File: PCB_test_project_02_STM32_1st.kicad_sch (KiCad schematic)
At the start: 12 parts

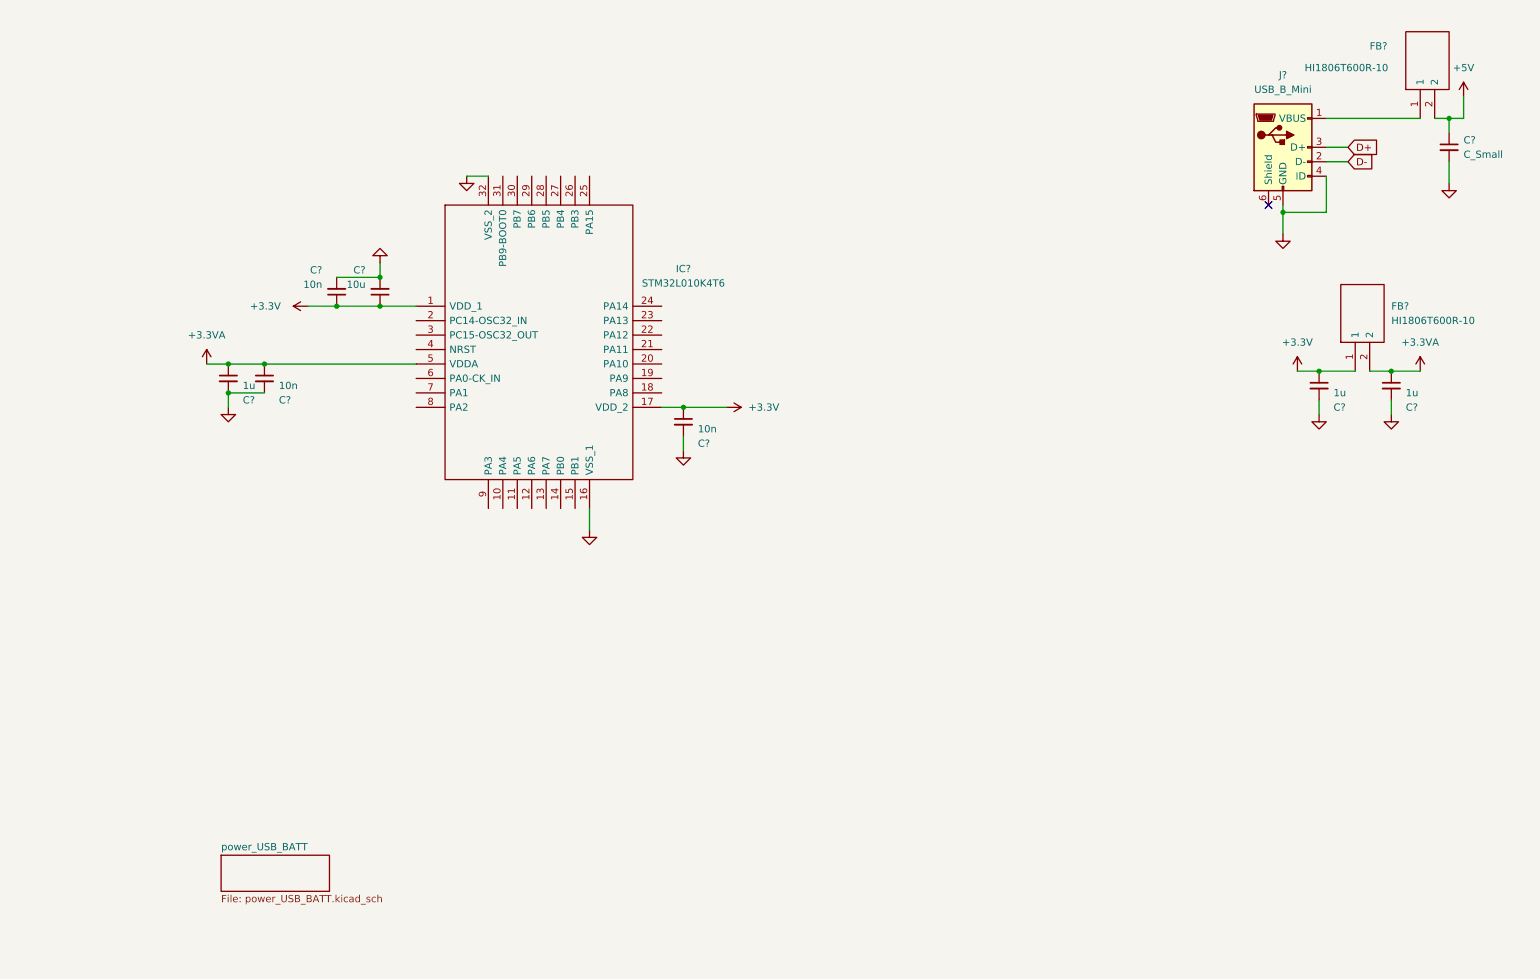
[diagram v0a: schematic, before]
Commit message: b
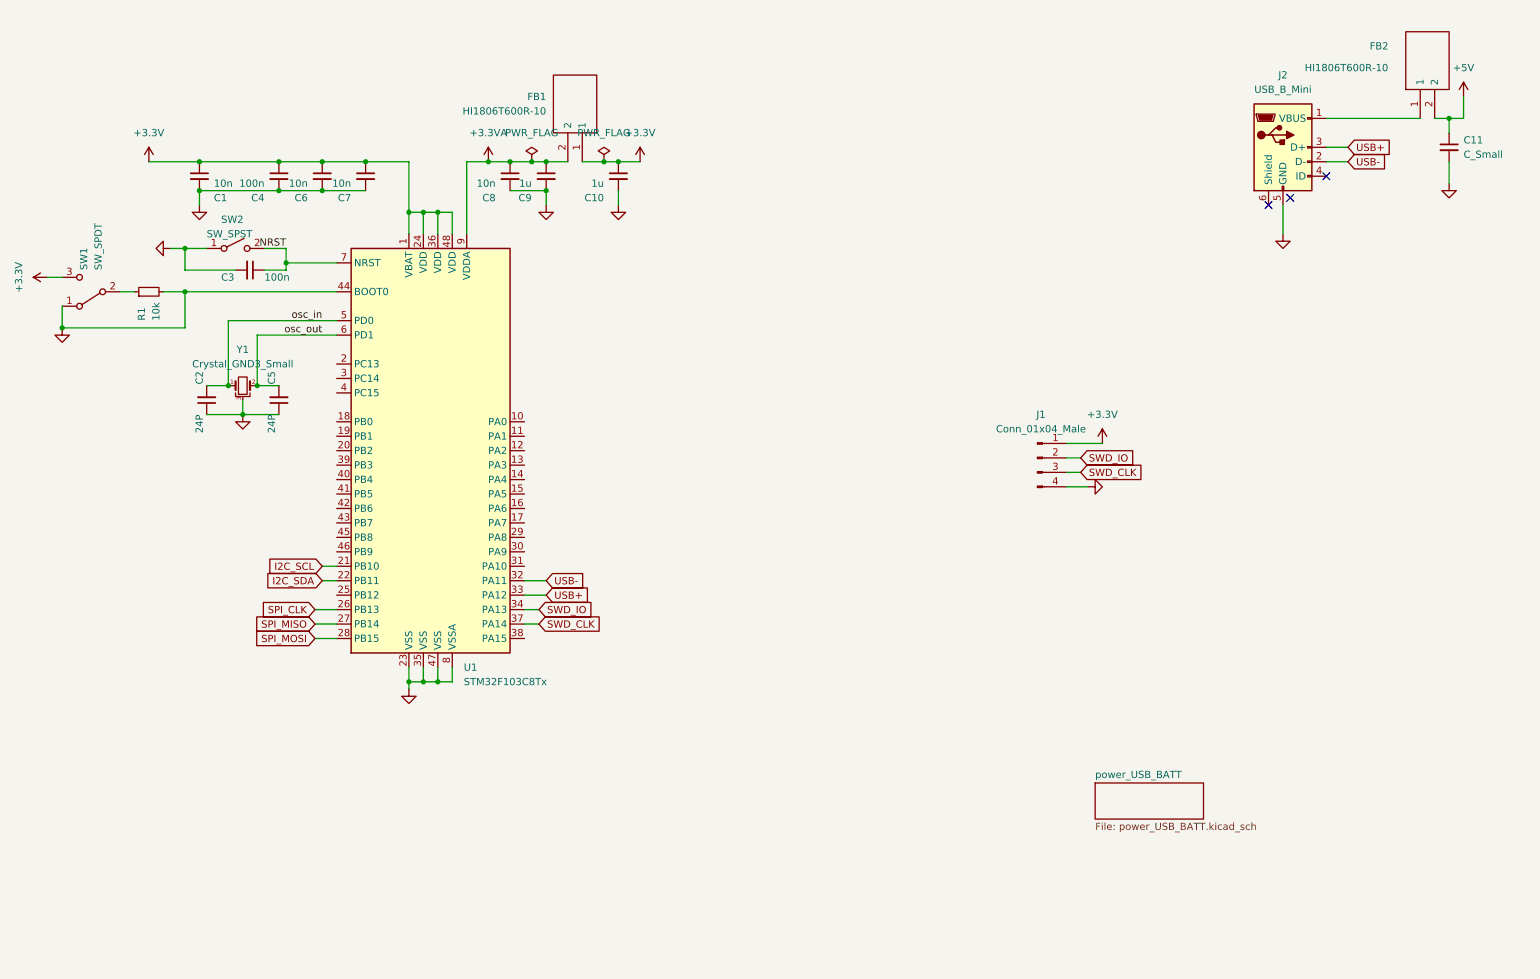
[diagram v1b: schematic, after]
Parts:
- removed C? (x2): 10n, symbol Device:C_Small
- removed C?: 10u, symbol Device:C_Small
- removed C?: 1u, symbol Device:C_Small
- removed IC?: STM32L010K4T6, QFP80P900X900X160-32N, symbol SamacSys_Parts:STM32L010K4T6
- added C1, C6, C7: 10n, symbol Device:C_Small
- added C2, C5: 24P, symbol Device:C_Small
- added C3, C4: 100n, symbol Device:C_Small
- added J1: Conn_01x04_Male, symbol Connector:Conn_01x04_Male
- added R1: 10k, symbol Device:R_Small
- added SW1: SW_SPDT, symbol Switch:SW_SPDT
- added SW2: SW_SPST, symbol Switch:SW_SPST
- added U1: STM32F103C8Tx, Package_QFP:LQFP-48_7x7mm_P0.5mm, symbol MCU_ST_STM32F1:STM32F103C8Tx
- added Y1: Crystal_GND3_Small, symbol Device:Crystal_GND3_Small
- gave numbers to parts that had none: 7
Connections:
- net +3.3VA: now also U1.9 (VDDA)
- net +3V3: now also C1.1, C4.1, C6.1, C7.1, J1.1 (Pin_1), SW1.3 (C), U1.1 (VBAT), U1.24 (VDD), U1.36 (VDD), U1.48 (VDD)
- net GND: now also C1.2, C2.1, C3.2, C4.2, C5.1, C6.2, C7.2, J1.4 (Pin_4), R1.2, SW1.1 (A), SW2.1 (A), U1.23 (VSS), U1.35 (VSS), U1.44 (BOOT0), U1.47 (VSS), U1.8 (VSSA), Y1.3; no longer J2.4 (ID)
- net D+ renamed USB+
- net USB+: now also U1.33 (PA12)
- net D- renamed USB-
- net USB-: now also U1.32 (PA11)
- new net: R1.1, SW1.2 (B)
- new net I2C_SCL: U1.21 (PB10)
- new net I2C_SDA: U1.22 (PB11)
- new net NRST: C3.1, SW2.2 (B), U1.7 (NRST)
- new net SPI_CLK: U1.26 (PB13)
- new net SPI_MISO: U1.27 (PB14)
- new net SPI_MOSI: U1.28 (PB15)
- new net SWD_CLK: J1.3 (Pin_3), U1.37 (PA14)
- new net SWD_IO: J1.2 (Pin_2), U1.34 (PA13)
- new net osc_in: C2.2, U1.5 (PD0), Y1.1
- new net osc_out: C5.2, U1.6 (PD1), Y1.2
- no-connect marks 1 -> 3
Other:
- moved on the sheet: C10, C8, C9, FB1

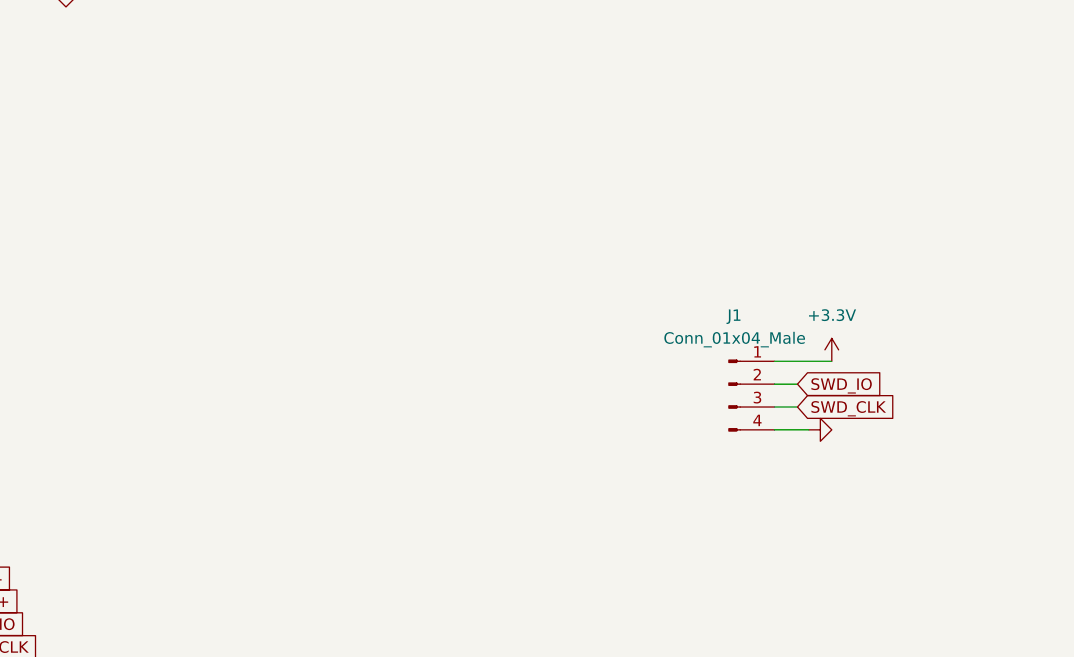
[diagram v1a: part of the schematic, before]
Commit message: y
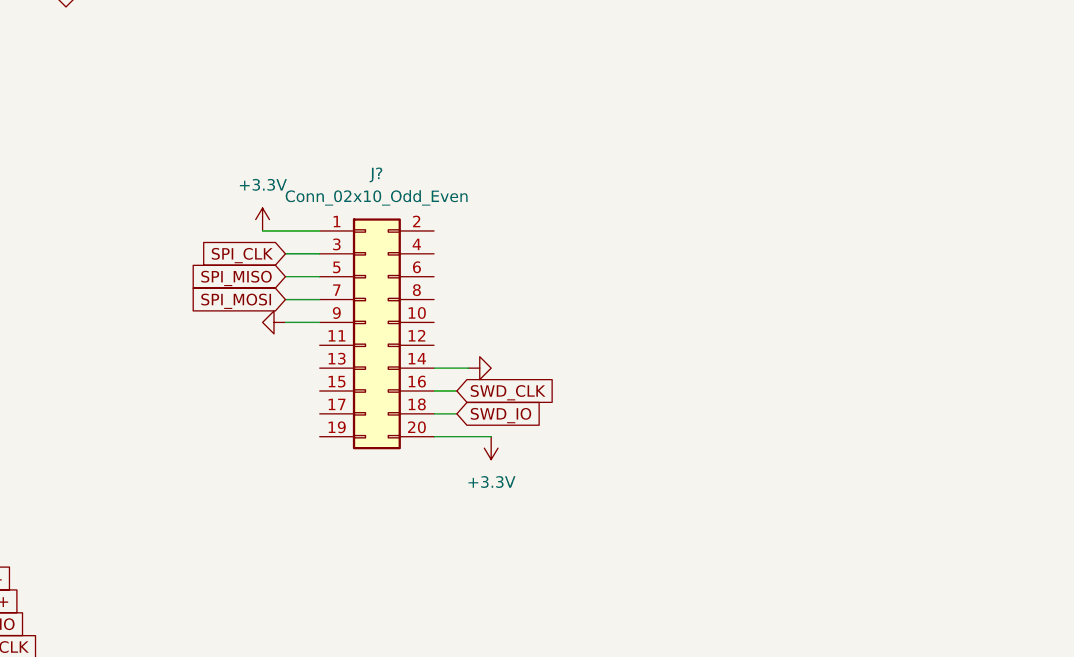
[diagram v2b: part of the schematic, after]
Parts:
- removed J1: Conn_01x04_Male, symbol Connector:Conn_01x04_Male
- added J?: Conn_02x10_Odd_Even, Connector_PinHeader_2.54mm:PinHeader_2x10_P2.54mm_Vertical, symbol Connector_Generic:Conn_02x10_Odd_Even
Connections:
- net +3V3: now also J?.1 (Pin_1), J?.20 (Pin_20)
- net GND: now also J?.14 (Pin_14), J?.9 (Pin_9)
- net SPI_CLK: now also J?.3 (Pin_3)
- net SPI_MISO: now also J?.5 (Pin_5)
- net SPI_MOSI: now also J?.7 (Pin_7)
- net SWD_CLK: now also J?.16 (Pin_16)
- net SWD_IO: now also J?.18 (Pin_18)

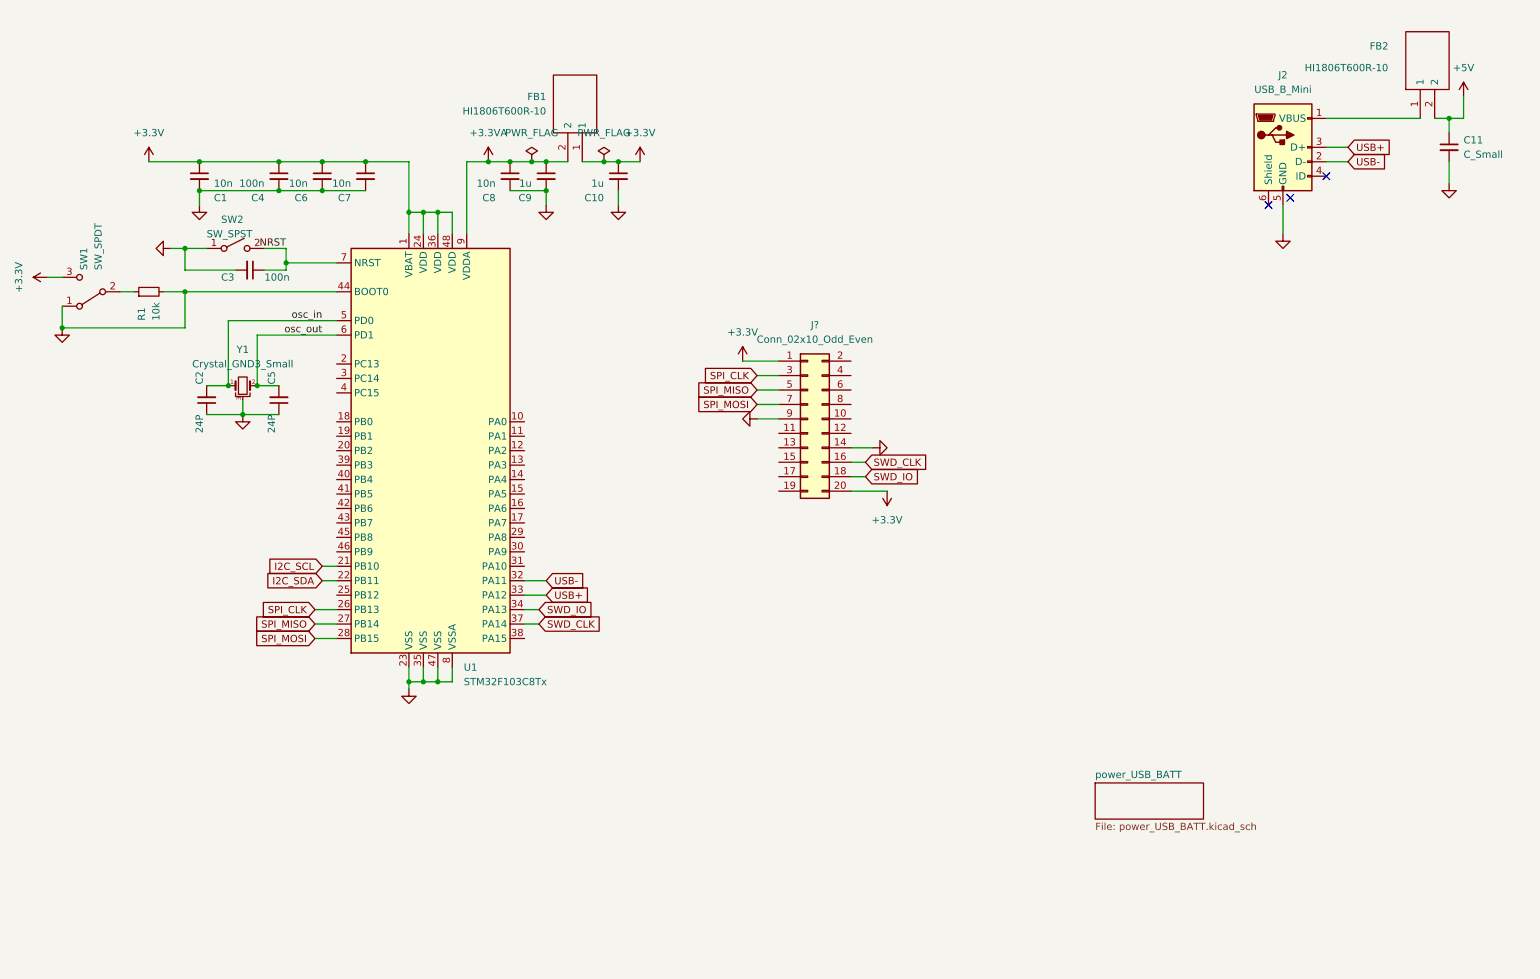
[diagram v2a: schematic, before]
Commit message: k
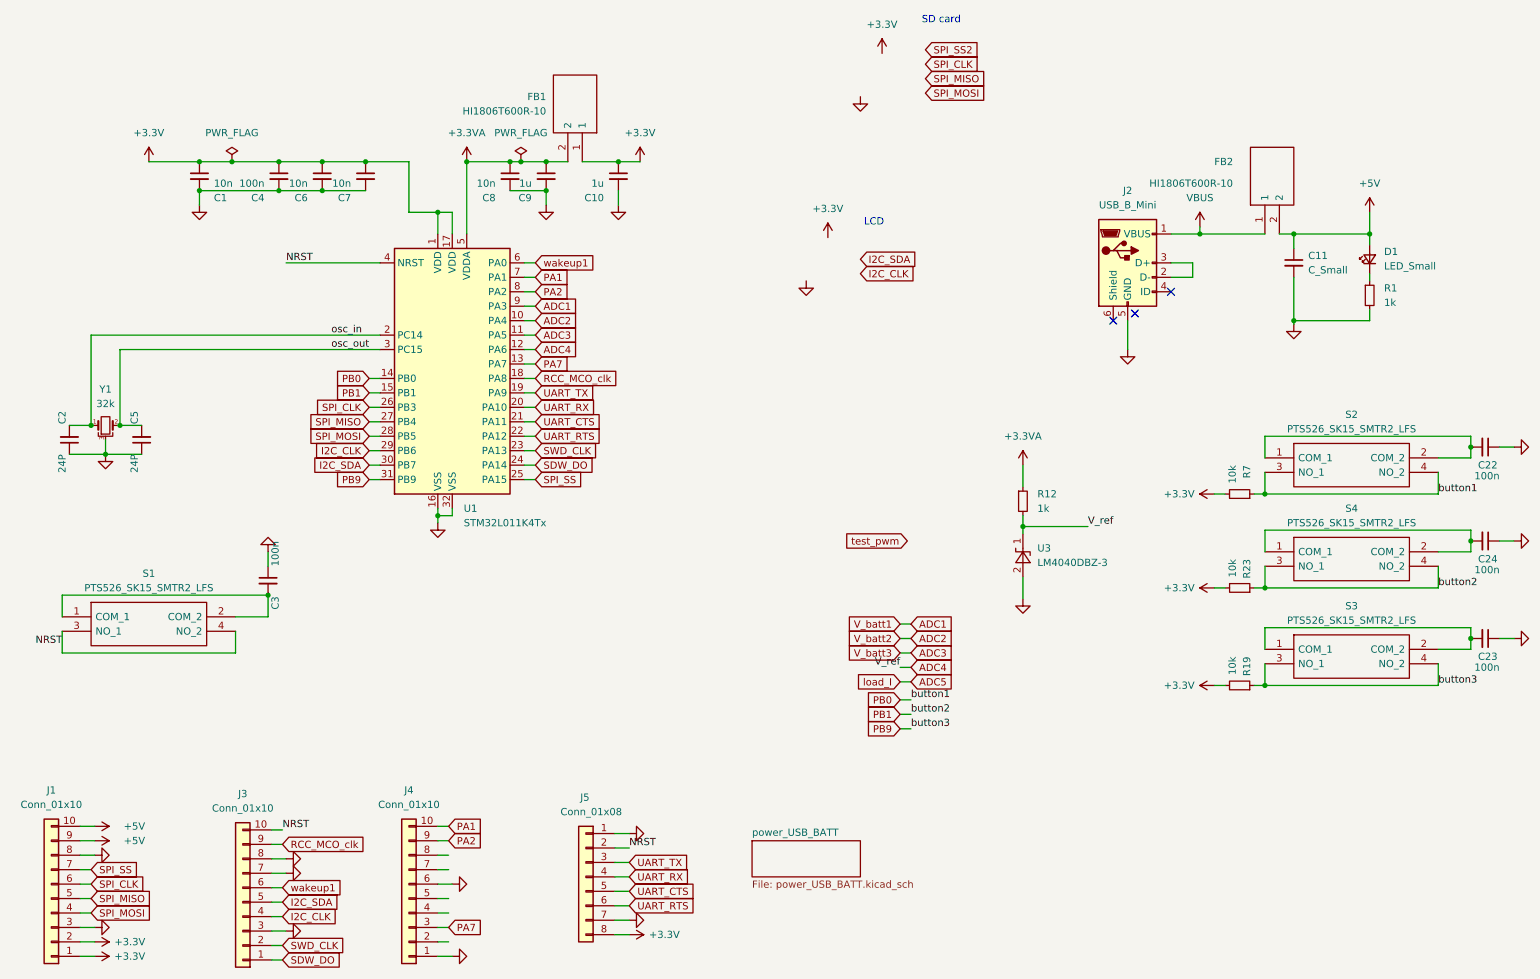
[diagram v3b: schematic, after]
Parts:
- removed J?: Conn_02x10_Odd_Even, Connector_PinHeader_2.54mm:PinHeader_2x10_P2.54mm_Vertical, symbol Connector_Generic:Conn_02x10_Odd_Even
- removed SW1: SW_SPDT, symbol Switch:SW_SPDT
- removed SW2: SW_SPST, symbol Switch:SW_SPST
- removed U1: STM32F103C8Tx, Package_QFP:LQFP-48_7x7mm_P0.5mm, symbol MCU_ST_STM32F1:STM32F103C8Tx
- added C22, C23, C24: 100n, Capacitor_SMD:C_0603_1608Metric_Pad1.08x0.95mm_HandSolder, symbol Device:C_Small
- added D1: LED_Small, LED_SMD:LED_0603_1608Metric_Pad1.05x0.95mm_HandSolder, symbol Device:LED_Small
- added J1, J3, J4: Conn_01x10, Connector_PinHeader_2.54mm:PinHeader_1x10_P2.54mm_Vertical, symbol Connector_Generic:Conn_01x10
- added J5: Conn_01x08, Connector_PinHeader_2.54mm:PinHeader_1x08_P2.54mm_Vertical, symbol Connector_Generic:Conn_01x08
- added R12: 1k, Resistor_SMD:R_0603_1608Metric_Pad0.98x0.95mm_HandSolder, symbol Device:R_Small
- added R19, R23, R7: 10k, Resistor_SMD:R_0603_1608Metric_Pad0.98x0.95mm_HandSolder, symbol Device:R_Small
- added S1, S2, S3, S4: PTS526_SK15_SMTR2_LFS, PTS526SK15SMTR2LFS, symbol SamacSys_Parts:PTS526_SK15_SMTR2_LFS
- added U1: STM32L011K4Tx, Package_QFP:LQFP-32_7x7mm_P0.8mm, symbol MCU_ST_STM32L0:STM32L011K4Tx
- added U3: LM4040DBZ-3, Package_TO_SOT_SMD:SOT-23, symbol Reference_Voltage:LM4040DBZ-3
- C1, C10, C11, C2, C3, C4, C5, C6, C7, C8, C9: footprint (none) -> Capacitor_SMD:C_0603_1608Metric_Pad1.08x0.95mm_HandSolder
- FB1, FB2: footprint BEADC4516X185N -> SamacSys_Parts:BEADC4516X185N
- R1: value 10k -> 1k; footprint (none) -> Resistor_SMD:R_0603_1608Metric_Pad0.98x0.95mm_HandSolder
- Y1: value Crystal_GND3_Small -> 32k
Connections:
- net USB- is gone; now on an unnamed net: J2.2 (D-)
- net +3.3VA: now also R12.1, U1.5 (VDDA)
- net +3V3: now also J1.1 (Pin_1), J1.2 (Pin_2), J5.8 (Pin_8), R19.2, R23.2, R7.2, U1.1 (VDD), U1.17 (VDD)
- net +5V: now also D1.2 (A), J1.10 (Pin_10), J1.9 (Pin_9)
- net GND: now also C3.1, C22.1, C23.1, C24.1, J1.3 (Pin_3), J1.8 (Pin_8), J3.3 (Pin_3), J3.7 (Pin_7), J3.8 (Pin_8), J4.1 (Pin_1), J4.6 (Pin_6), J5.1 (Pin_1), J5.7 (Pin_7), U1.16 (VSS), U1.32 (VSS), U3.2 (A); no longer C3.2
- net I2C_SDA: now also J3.5 (Pin_5), U1.30 (PB7)
- net NRST: now also J3.10 (Pin_10), J5.2 (Pin_2), S1.3 (NO_1), S1.4 (NO_2), U1.4 (NRST); no longer C3.1
- net SPI_CLK: now also J1.6 (Pin_6), U1.26 (PB3)
- net SPI_MISO: now also J1.5 (Pin_5), U1.27 (PB4)
- net SPI_MOSI: now also J1.4 (Pin_4), U1.28 (PB5)
- net SWD_CLK: now also J3.2 (Pin_2), U1.23 (PA13)
- net osc_in: now also U1.2 (PC14)
- net osc_out: now also U1.3 (PC15)
- net VBUS: now reaches FB2.1, J2.1 (VBUS)
- net at R1.1: now also D1.1 (K)
- net USB+: no longer names the net of J2.3 (D+)
- new net: C22.2, S2.1 (COM_1), S2.2 (COM_2)
- new net: C3.2, S1.1 (COM_1), S1.2 (COM_2)
- new net: C24.2, S4.1 (COM_1), S4.2 (COM_2)
- new net: C23.2, S3.1 (COM_1), S3.2 (COM_2)
- new net ADC1: U1.9 (PA3)
- new net ADC2: U1.10 (PA4)
- new net ADC3: U1.11 (PA5)
- new net ADC4: R12.2, U1.12 (PA6), U3.1 (K)
- new net I2C_CLK: J3.4 (Pin_4), U1.29 (PB6)
- new net PA1: J4.10 (Pin_10), U1.7 (PA1)
- new net PA2: J4.9 (Pin_9), U1.8 (PA2)
- new net PA7: J4.3 (Pin_3), U1.13 (PA7)
- new net PB0: R7.1, S2.3 (NO_1), S2.4 (NO_2), U1.14 (PB0)
- new net PB1: R23.1, S4.3 (NO_1), S4.4 (NO_2), U1.15 (PB1)
- new net PB9: R19.1, S3.3 (NO_1), S3.4 (NO_2), U1.31 (PB9)
- new net RCC_MCO_clk: J3.9 (Pin_9), U1.18 (PA8)
- new net SDW_DO: J3.1 (Pin_1), U1.24 (PA14)
- new net SPI_SS: J1.7 (Pin_7), U1.25 (PA15)
- new net UART_CTS: J5.5 (Pin_5), U1.21 (PA11)
- new net UART_RTS: J5.6 (Pin_6), U1.22 (PA12)
- new net UART_RX: J5.4 (Pin_4), U1.20 (PA10)
- new net UART_TX: J5.3 (Pin_3), U1.19 (PA9)
- new net wakeup1: J3.6 (Pin_6), U1.6 (PA0)
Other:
- note added: "LCD"
- note added: "SD card"
- moved on the sheet: C11, C2, C3, C5, FB2, J2, Y1
